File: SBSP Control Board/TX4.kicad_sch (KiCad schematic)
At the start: 13 parts, among them U6 ADAR1000ACCZN

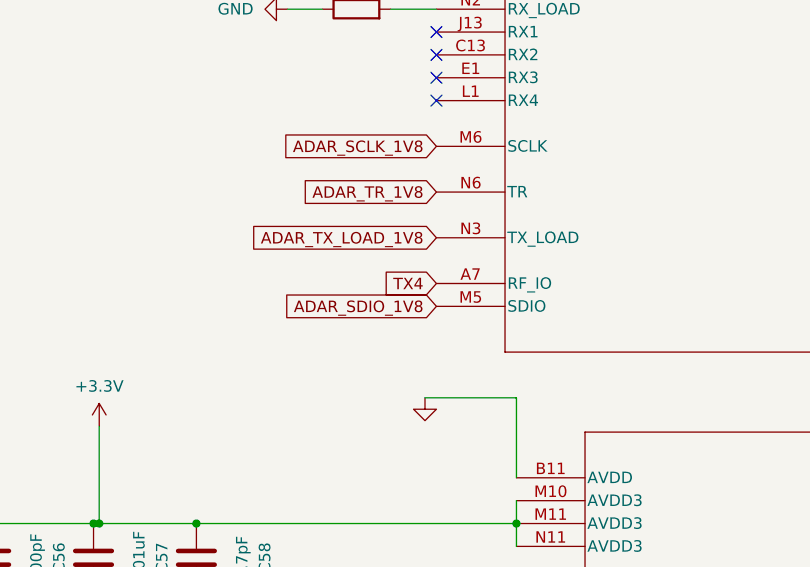
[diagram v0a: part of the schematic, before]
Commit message: first rev of trans. line routed
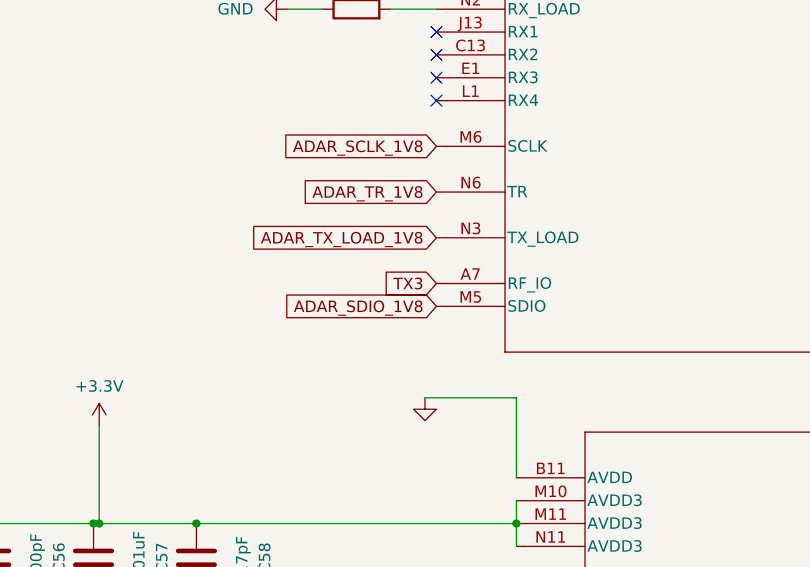
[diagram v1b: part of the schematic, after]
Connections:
- net TX4 renamed TX3
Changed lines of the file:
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@@
 		)
 	)
-	(global_label "TX4"
+	(global_label "TX3"
 		(shape input)
 		(at 152.4 119.38 180)

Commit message: 'finished' the first IC routing
need to re do and see what connections we need to make for programming. also need to see about better ground connections to the IC.
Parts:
- C39, C40, C41, C42, C43, C44, C45, C46, C56, C57, C58: footprint Capacitor_SMD:C_1206_3216Metric -> Resistor_SMD:R_0603_1608Metric
- R15: footprint Resistor_SMD:R_1206_3216Metric -> Resistor_SMD:R_0603_1608Metric
- U6: footprint CC-88-1_ADI -> adar1000:CC-88-1_ADI
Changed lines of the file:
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@@
 			)
 		)
-		(property "Footprint" "Capacitor_SMD:C_1206_3216Metric"
+		(property "Footprint" "Resistor_SMD:R_0603_1608Metric"
 			(at 169.8752 180.34 0)
 			(hide yes)
@@
 			)
 		)
-		(property "Footprint" "Capacitor_SMD:C_1206_3216Metric"
+		(property "Footprint" "Resistor_SMD:R_0603_1608Metric"
 			(at 221.9452 180.34 0)
 			(hide yes)
@@
 			)
 		)
-		(property "Footprint" "Resistor_SMD:R_1206_3216Metric"
+		(property "Footprint" "Resistor_SMD:R_0603_1608Metric"
 			(at 143.51 90.678 90)
 			(hide yes)
@@
 			)
 		)
-		(property "Footprint" "Capacitor_SMD:C_1206_3216Metric"
+		(property "Footprint" "Resistor_SMD:R_0603_1608Metric"
 			(at 126.6952 153.67 0)
 			(hide yes)
@@
 			)
 		)
-		(property "Footprint" "CC-88-1_ADI"
+		(property "Footprint" "adar1000:CC-88-1_ADI"
 			(at 173.99 240.03 0)
 			(hide yes)
@@
 			)
 		)
-		(property "Footprint" "Capacitor_SMD:C_1206_3216Metric"
+		(property "Footprint" "Resistor_SMD:R_0603_1608Metric"
 			(at 157.1752 180.34 0)
 			(hide yes)
@@
 			)
 		)
-		(property "Footprint" "Capacitor_SMD:C_1206_3216Metric"
+		(property "Footprint" "Resistor_SMD:R_0603_1608Metric"
 			(at 195.2752 180.34 0)
 			(hide yes)
@@
 			)
 		)
-		(property "Footprint" "Capacitor_SMD:C_1206_3216Metric"
+		(property "Footprint" "Resistor_SMD:R_0603_1608Metric"
 			(at 143.2052 180.34 0)
 			(hide yes)
@@
 			)
 		)
-		(property "Footprint" "Capacitor_SMD:C_1206_3216Metric"
+		(property "Footprint" "Resistor_SMD:R_0603_1608Metric"
 			(at 182.5752 180.34 0)
 			(hide yes)
@@
 			)
 		)
-		(property "Footprint" "CC-88-1_ADI"
+		(property "Footprint" "adar1000:CC-88-1_ADI"
 			(at 152.4 58.42 0)
 			(hide yes)
@@
 			)
 		)
-		(property "Footprint" "Capacitor_SMD:C_1206_3216Metric"
+		(property "Footprint" "Resistor_SMD:R_0603_1608Metric"
 			(at 130.5052 180.34 0)
 			(hide yes)
@@
 			)
 		)
-		(property "Footprint" "Capacitor_SMD:C_1206_3216Metric"
+		(property "Footprint" "Resistor_SMD:R_0603_1608Metric"
 			(at 103.8352 153.67 0)
 			(hide yes)
@@
 			)
 		)
-		(property "Footprint" "Capacitor_SMD:C_1206_3216Metric"
+		(property "Footprint" "Resistor_SMD:R_0603_1608Metric"
 			(at 209.2452 180.34 0)
 			(hide yes)
@@
 			)
 		)
-		(property "Footprint" "CC-88-1_ADI"
+		(property "Footprint" "adar1000:CC-88-1_ADI"
 			(at 161.29 140.97 0)
 			(hide yes)
@@
 			)
 		)
-		(property "Footprint" "Capacitor_SMD:C_1206_3216Metric"
+		(property "Footprint" "Resistor_SMD:R_0603_1608Metric"
 			(at 115.2652 153.67 0)
 			(hide yes)
